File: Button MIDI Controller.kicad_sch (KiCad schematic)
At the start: 33 parts, among them J1 SWD, J2 USB_C_Receptacle_USB2.0_16P, U1 RP2040, U2 W25Q16JVZPIQ, U3 USBLC6-2SC6, U4 XC6206PxxxMR, Y1 X322512MSB4SI

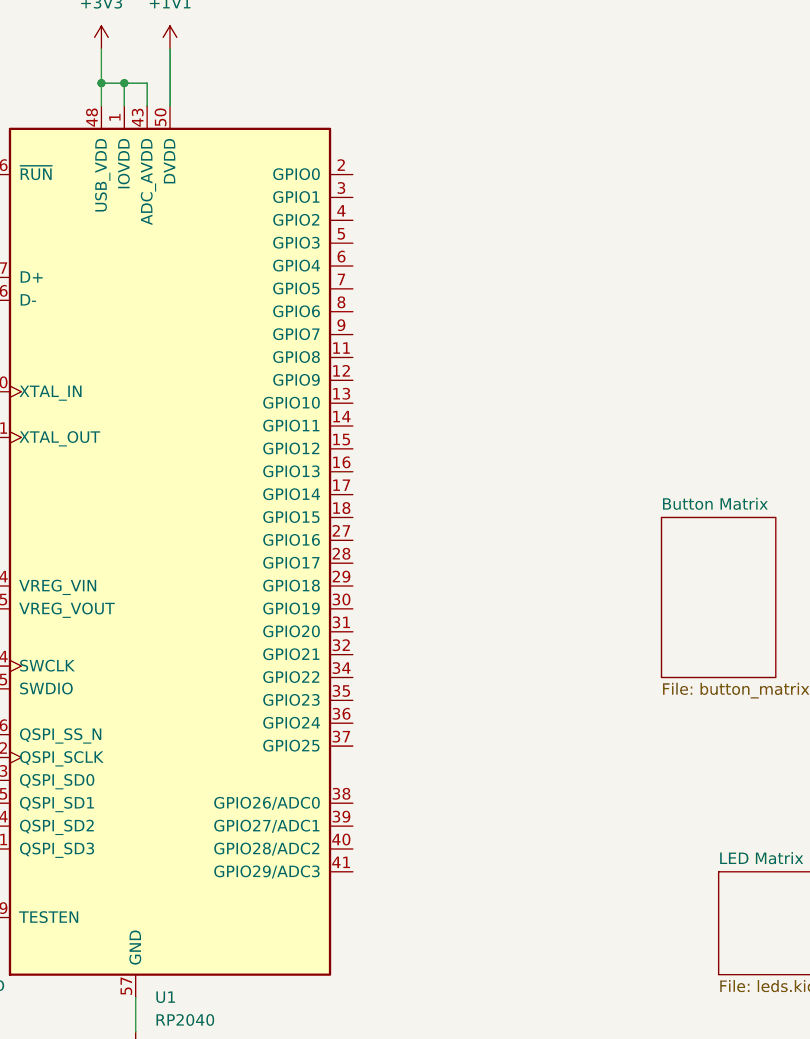
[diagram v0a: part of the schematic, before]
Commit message: updates
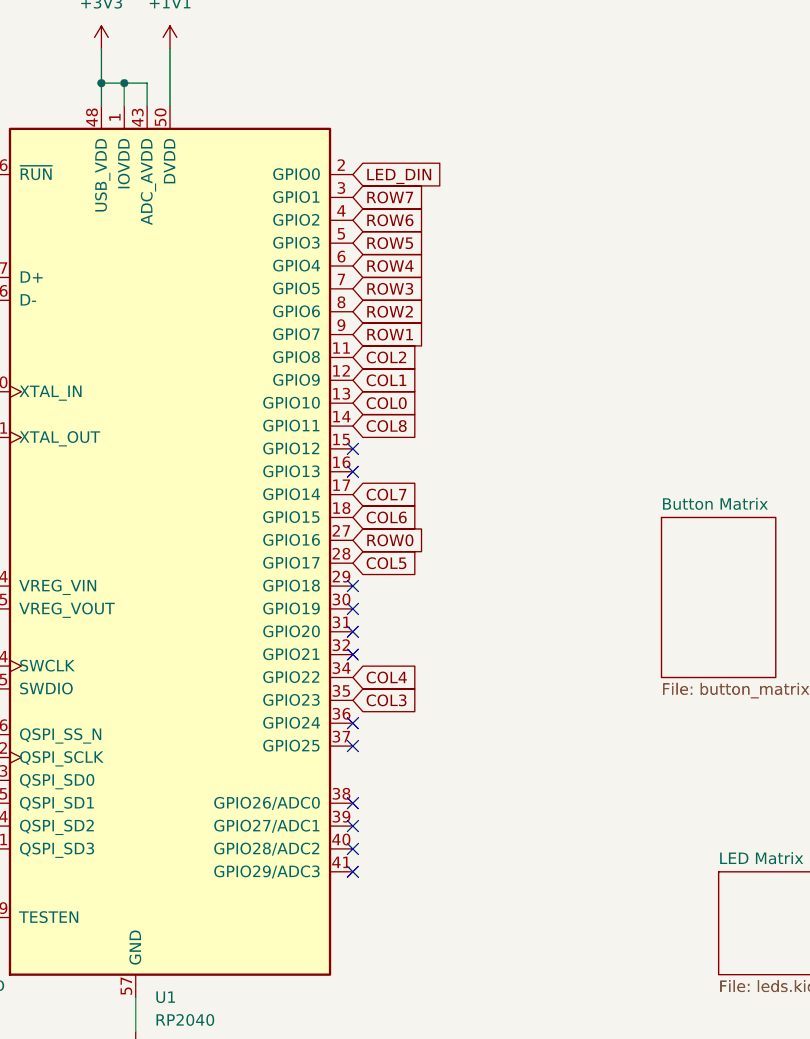
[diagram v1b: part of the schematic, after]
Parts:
- C1, C10, C11, C12, C13, C14, C15, C16, C17, C2, C3, C4, C5, C6, C7, C8, C9: footprint Capacitor_SMD:C_0603_1608Metric -> Capacitor_SMD:C_0402_1005Metric-notxt
- F1: footprint Fuse:Fuse_0603_1608Metric -> Fuse:Fuse_0402_1005Metric-notxt
- J1: footprint Connector_PinHeader_1.00mm:PinHeader_1x05_P1.00mm_Vertical_SMD_Pin1Right -> Connector_PinHeader_1.00mm:PinHeader_1x05_P1.00mm_Vertical_SMD_Pin1Right-notxt
- J2: footprint Connector_USB:USB_C_Receptacle_G-Switch_GT-USB-7025 -> Connector_USB:USB_C_Receptacle_G-Switch_GT-USB-7025-notxt
- R1, R2, R3, R4, R5, R6, R7: footprint Resistor_SMD:R_0603_1608Metric -> Resistor_SMD:R_0402_1005Metric-notext
- TP1: footprint TestPoint:TestPoint_Pad_4.0x4.0mm -> TestPoint:TestPoint_Pad_1.0x1.0mm-notxt
- U1: footprint Footprints:RP2040-QFN-56 -> Footprints:RP2040-QFN-56-notext
- U2: footprint W25Q16JVZPIQ:SON127P500X600X80-9N -> W25Q16JVZPIQ:SON127P500X600X80-9N-notxt
- U3: footprint Package_TO_SOT_SMD:SOT-23-6 -> Package_TO_SOT_SMD:SOT-23-6-notxt
- U4: footprint Package_TO_SOT_SMD:SOT-23-3 -> Package_TO_SOT_SMD:SOT-23-3-notxt
- Y1: footprint Crystal:Crystal_SMD_7050-4Pin_7.0x5.0mm -> Crystal:Crystal_SMD_2016-4Pin_2.0x1.6mm-notxt
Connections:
- net COL2: now reaches U1.11 (GPIO8)
- net COL1: now reaches U1.12 (GPIO9)
- net COL0: now reaches U1.13 (GPIO10)
- net COL8: now reaches U1.14 (GPIO11)
- net COL7: now reaches U1.17 (GPIO14)
- net COL6: now reaches U1.18 (GPIO15)
- net LED_DIN: now reaches U1.2 (GPIO0)
- net ROW0: now reaches U1.27 (GPIO16)
- net COL5: now reaches U1.28 (GPIO17)
- net ROW7: now reaches U1.3 (GPIO1)
- net COL4: now reaches U1.34 (GPIO22)
- net COL3: now reaches U1.35 (GPIO23)
- net ROW6: now reaches U1.4 (GPIO2)
- net ROW5: now reaches U1.5 (GPIO3)
- net ROW4: now reaches U1.6 (GPIO4)
- net ROW3: now reaches U1.7 (GPIO5)
- net ROW2: now reaches U1.8 (GPIO6)
- net ROW1: now reaches U1.9 (GPIO7)
- no-connect marks 2 -> 14

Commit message: yeah have some updates my g
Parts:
- C1, C2: JLCPCB Part (none) -> C541361
- C10, C11, C12, C13, C14, C15, C3, C7, C8, C9: JLCPCB Part (none) -> C541407
- C16, C4, C5, C6: JLCPCB Part (none) -> C437522
- C17: JLCPCB Part (none) -> C6119763
- F1: JLCPCB Part (none) -> C136320
- J1, TP1: now left out of the parts list
- J2: JLCPCB Part (none) -> C963213
- R1, R2, R5: JLCPCB Part (none) -> C11702
- R3, R4: JLCPCB Part (none) -> C25100
- R6, R7: JLCPCB Part (none) -> C25905
- U1: JLCPCB Part (none) -> C2040
- U2: JLCPCB Part (none) -> C377853
- U3: JLCPCB Part (none) -> C7519
- U4: JLCPCB Part (none) -> C5148692
- Y1: JLCPCB Part (none) -> C9002

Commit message: updates
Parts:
- F1: footprint Fuse:Fuse_0402_1005Metric-notxt -> Fuse:Fuse_1206_3216Metric
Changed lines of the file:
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@@
 			)
 		)
-		(property "Footprint" "Fuse:Fuse_0402_1005Metric-notxt"
+		(property "Footprint" "Fuse:Fuse_1206_3216Metric"
 			(at 199.39 113.03 0)
 			(effects

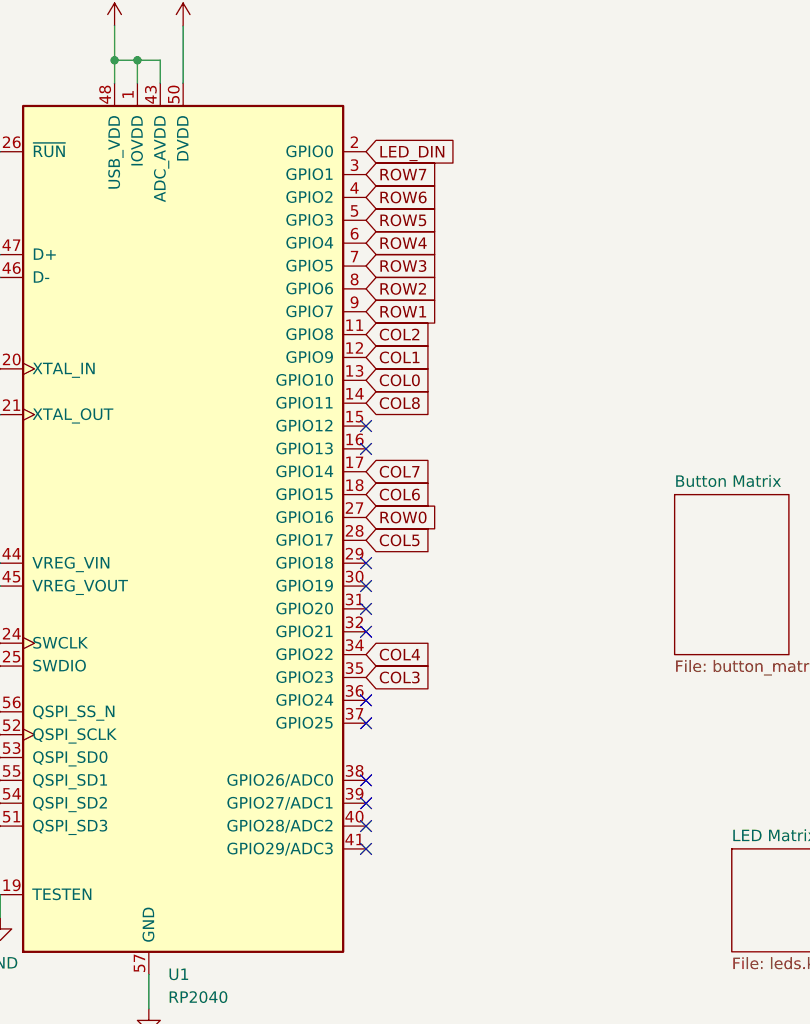
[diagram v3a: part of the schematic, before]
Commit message: boardstar updates & me ruining it
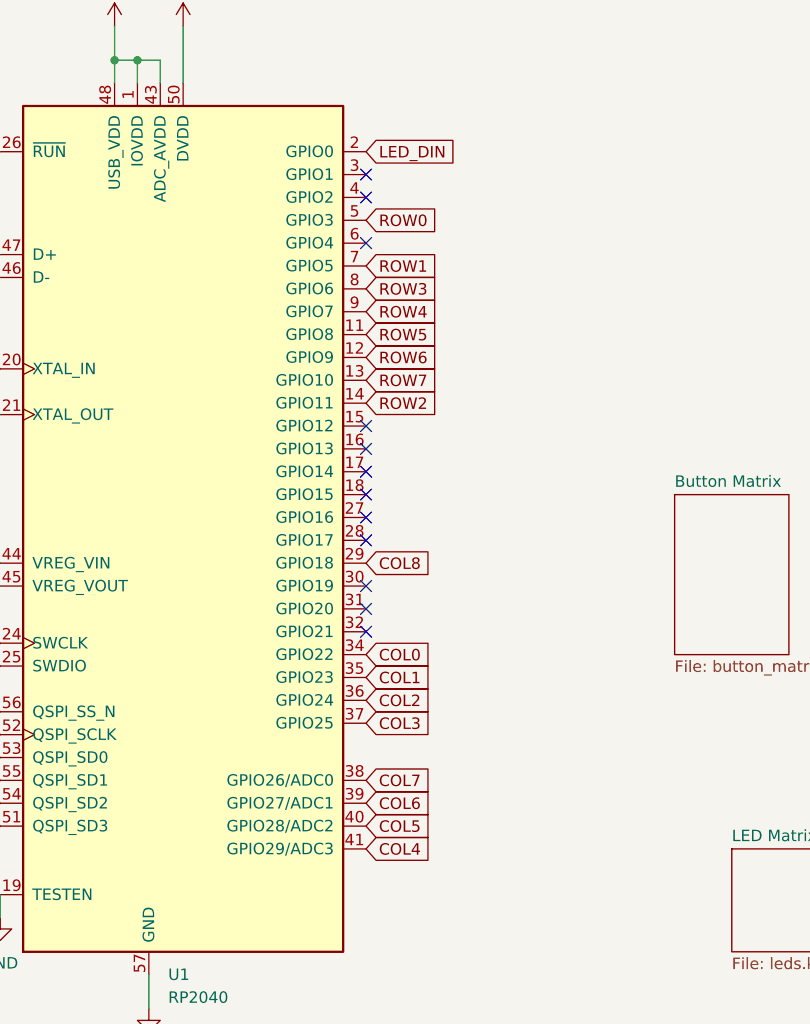
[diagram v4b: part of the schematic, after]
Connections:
- net COL0: now also U1.34 (GPIO22); no longer U1.13 (GPIO10)
- net COL1: now also U1.35 (GPIO23); no longer U1.12 (GPIO9)
- net COL2: now also U1.36 (GPIO24); no longer U1.11 (GPIO8)
- net COL3: now also U1.37 (GPIO25); no longer U1.35 (GPIO23)
- net COL4: now also U1.41 (GPIO29/ADC3); no longer U1.34 (GPIO22)
- net COL5: now also U1.40 (GPIO28/ADC2); no longer U1.28 (GPIO17)
- net COL6: now also U1.39 (GPIO27/ADC1); no longer U1.18 (GPIO15)
- net COL7: now also U1.38 (GPIO26/ADC0); no longer U1.17 (GPIO14)
- net COL8: now also U1.29 (GPIO18); no longer U1.14 (GPIO11)
- net ROW0: now also U1.5 (GPIO3); no longer U1.27 (GPIO16)
- net ROW1: now also U1.7 (GPIO5); no longer U1.9 (GPIO7)
- net ROW2: now also U1.14 (GPIO11); no longer U1.8 (GPIO6)
- net ROW3: now also U1.8 (GPIO6); no longer U1.7 (GPIO5)
- net ROW4: now also U1.9 (GPIO7); no longer U1.6 (GPIO4)
- net ROW5: now also U1.11 (GPIO8); no longer U1.5 (GPIO3)
- net ROW6: now also U1.12 (GPIO9); no longer U1.4 (GPIO2)
- net ROW7: now also U1.13 (GPIO10); no longer U1.3 (GPIO1)
